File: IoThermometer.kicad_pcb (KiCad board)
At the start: 2 copper layers, 82.6 x 33 mm, 11 parts, among them U1 NodeMCU_Amica_R2

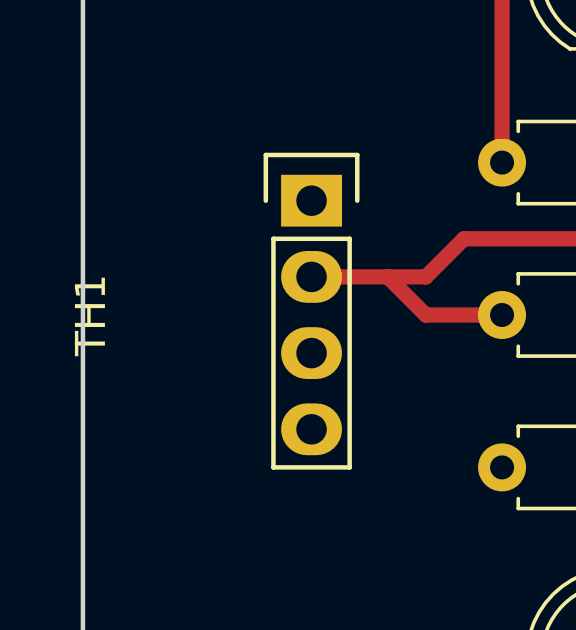
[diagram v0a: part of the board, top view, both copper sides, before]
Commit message: adjust layer visibility
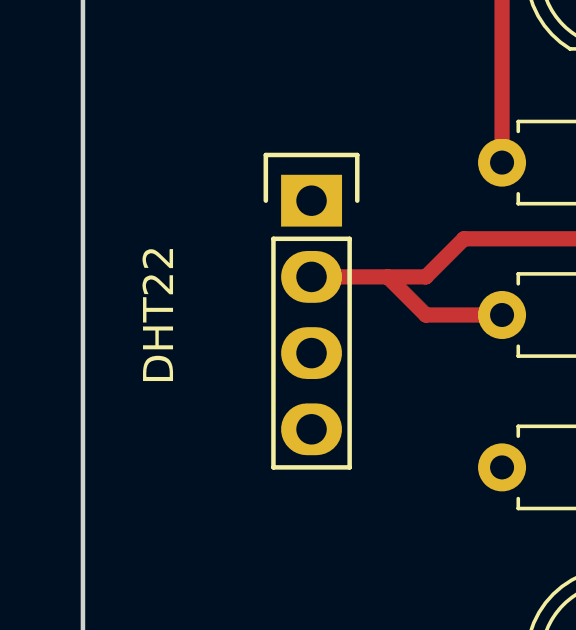
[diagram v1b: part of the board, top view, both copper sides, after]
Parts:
- renumbered TH1 to DHT22
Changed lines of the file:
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@@
   )
   (layers
-    (0 F.Cu signal)
-    (31 B.Cu signal)
-    (32 B.Adhes user)
-    (33 F.Adhes user)
-    (34 B.Paste user)
-    (35 F.Paste user)
+    (0 F.Cu signal hide)
+    (31 B.Cu signal hide)
+    (32 B.Adhes user hide)
+    (33 F.Adhes user hide)
+    (34 B.Paste user hide)
+    (35 F.Paste user hide)
     (36 B.SilkS user)
-    (37 F.SilkS user hide)
+    (37 F.SilkS user)
     (38 B.Mask user)
     (39 F.Mask user)
@@
       (effects (font (size 1 1) (thickness 0.15)))
     )
-    (fp_text value LED (at 1.27 3.96 90) (layer F.Fab)
+    (fp_text value LED (at 2.54 -5.08 90) (layer F.Fab)
       (effects (font (size 1 1) (thickness 0.15)))
     )
@@
       (effects (font (size 1 1) (thickness 0.15)))
     )
-    (fp_text value LED (at 1.27 3.96 90) (layer F.Fab)
+    (fp_text value LED (at -1.27 -5.08 90) (layer F.Fab)
       (effects (font (size 1 1) (thickness 0.15)))
     )
@@
   (module Sensors:DHT22_Temperature_Humidity (layer F.Cu)
     (at 112.84 107.57 270)
-    (fp_text reference TH1 (at 0 7.35 90) (layer F.SilkS)
+    (fp_text reference DHT22 (at 0 5.08 90) (layer F.SilkS)
       (effects (font (size 1 1) (thickness 0.15)))
     )
@@
   (segment (start 116.65 107.57) (end 115.38 106.3) (width 0.508) (layer F.Cu) (net 25))
   (segment (start 119.19 107.57) (end 116.65 107.57) (width 0.508) (layer F.Cu) (net 25))
-  (zone (net 2) (net_name GND) (layer B.Cu) (hatch edge 0.508)
+  (zone (net 4) (net_name +3V3) (layer F.Cu) (hatch edge 0.508)
     (connect_pads (clearance 0.508))
     (min_thickness 0.254)
@@
     )
   )
-  (zone (net 4) (net_name +3V3) (layer F.Cu) (hatch edge 0.508)
+  (zone (net 2) (net_name GND) (layer B.Cu) (hatch edge 0.508)
     (connect_pads (clearance 0.508))
     (min_thickness 0.254)
